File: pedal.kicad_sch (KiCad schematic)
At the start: 46 parts, among them J1 Conn_01x03_Socket, J2 Conn_01x01_Pin, J3 Conn_01x01_Pin, J4 Conn_01x01_Pin, J5 Conn_01x01_Pin, J6 Conn_01x02_Socket, SW1 EG5498-ND, SW2 SW_SPDT, SW3 EG5498-ND, T1 142B, U1 TL084

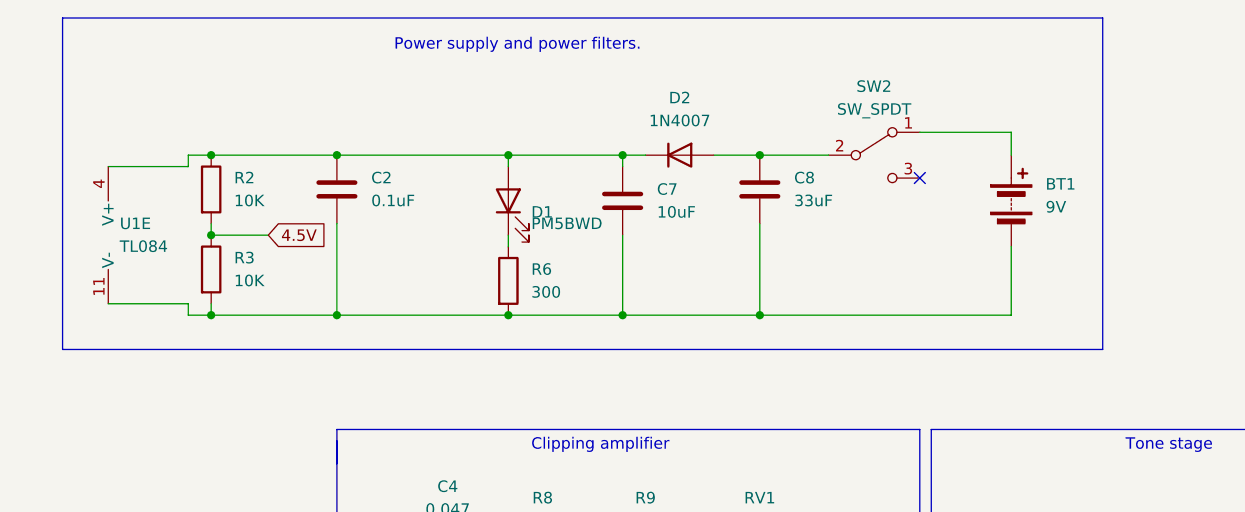
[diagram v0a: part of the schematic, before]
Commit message: Add files via upload
Fixed some small errors.
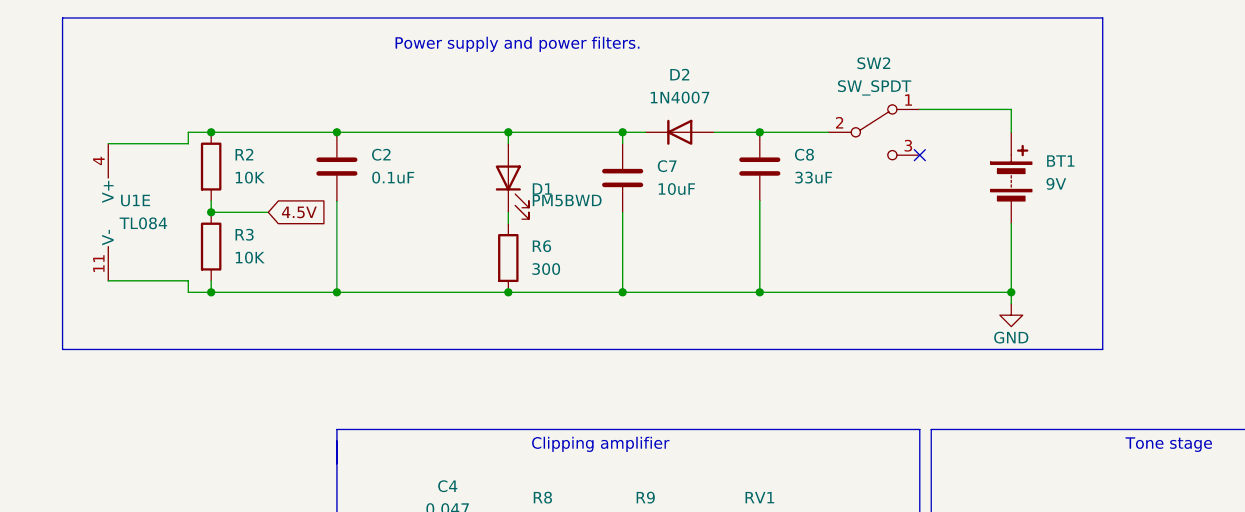
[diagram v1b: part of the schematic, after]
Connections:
- net GND: now also BT1.2 (-), C2.2, C7.2, C8.2, R3.2, R6.2, U1.11 (V-)
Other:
- moved on the sheet: BT1, C2, C7, C8, D1, D2, R2, R3, R6, SW2, U1E
